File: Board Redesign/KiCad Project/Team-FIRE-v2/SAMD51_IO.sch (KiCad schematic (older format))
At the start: 20 parts, among them SW1 RESET, U5 SAMD51, U6 AT25DF041x-UxN-x, Y1 32.768kHz

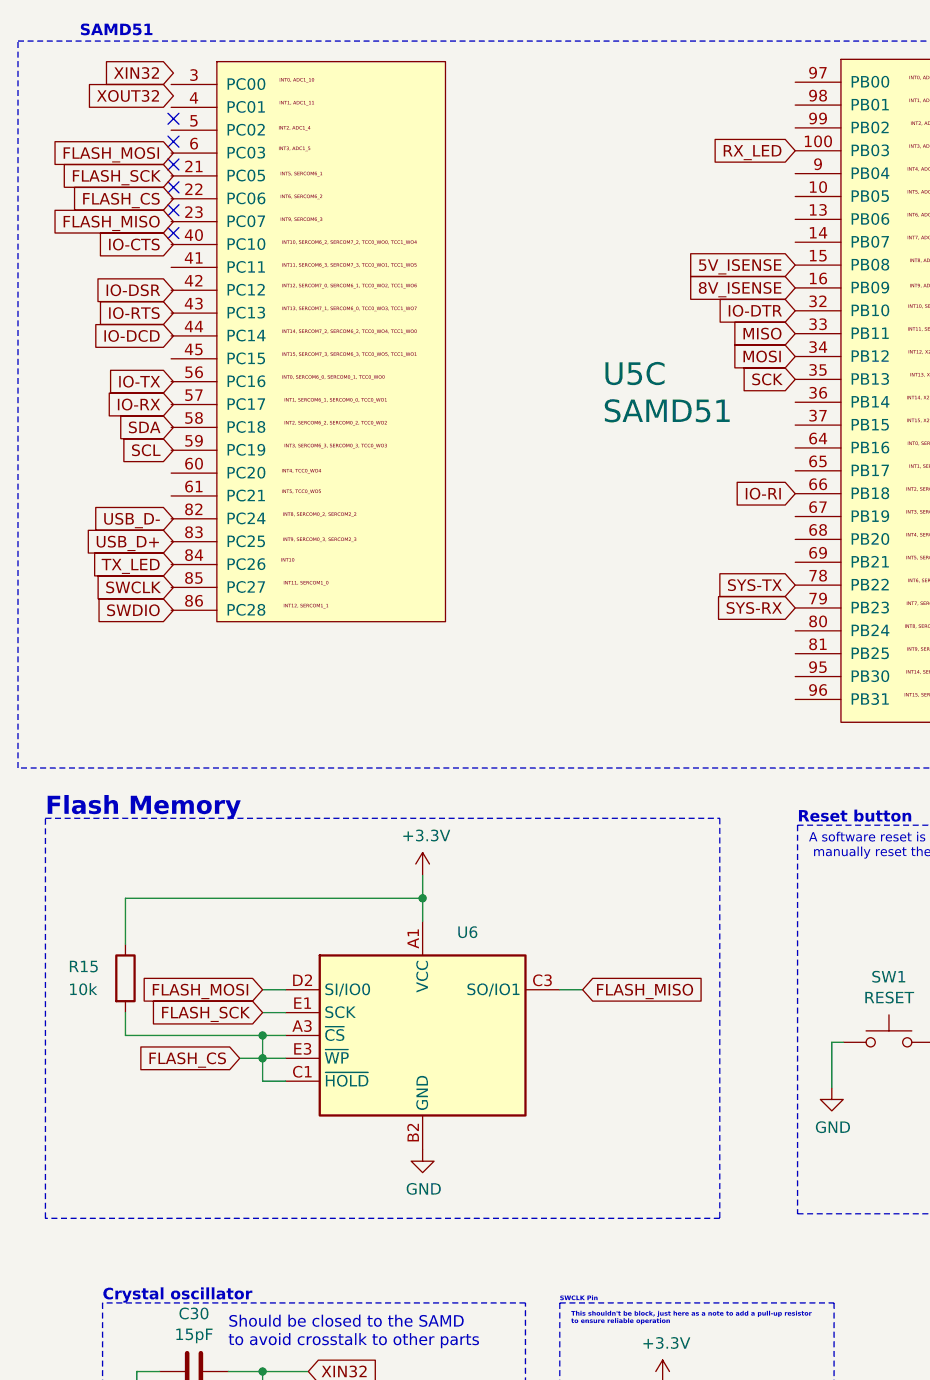
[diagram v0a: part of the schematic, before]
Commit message: Fixed some stuff (woops)
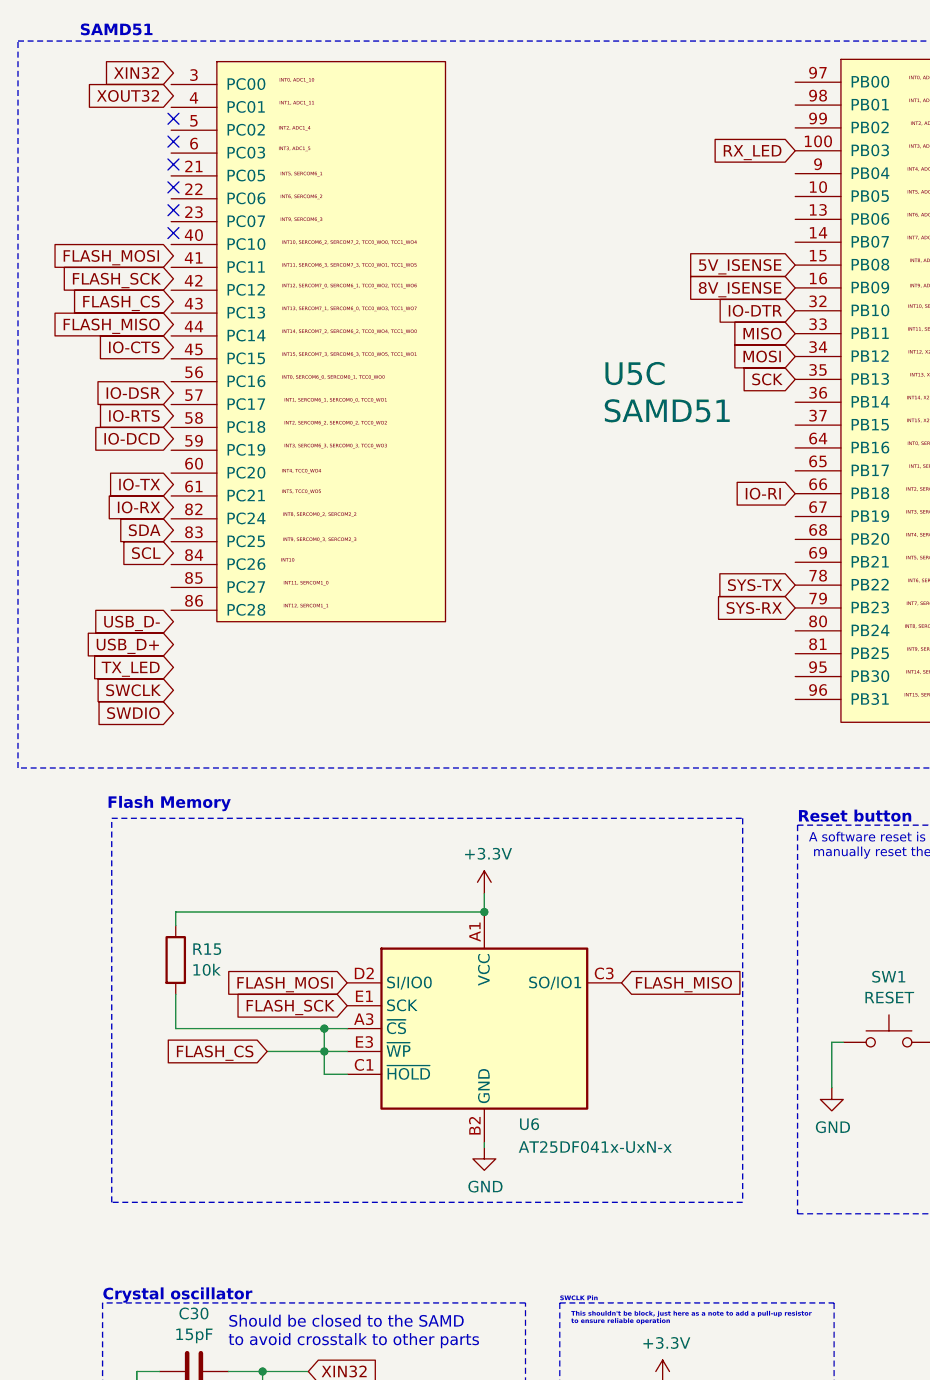
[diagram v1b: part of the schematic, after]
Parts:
- R15: footprint Resistor_SMD:R_0603_1608Metric -> (none); Link https://www.mouser.com/ProductDetail/Vishay-Beyschlag/MCT06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 -> (none); MPN MCT06030E1002BP100 -> (none); Manufacturer Vishay -> (none); Supplier Mouser -> (none); Supplier PN 594-MCT06030E1002BP1 -> (none); Tolerance 0.1% -> (none); Type Thin Film Resistor -> (none); Voltage Rating 75 V -> (none)
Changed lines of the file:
@@
 Comment4 ""
 $EndDescr
+Text GLabel 1260 3190 0    50   Input ~ 0
+USB_D-
+Text GLabel 1260 3290 0    50   Input ~ 0
+USB_D+
+Text GLabel 1260 2790 0    50   Input ~ 0
+SDA
+Text GLabel 1260 2890 0    50   Input ~ 0
+SCL
 $Comp
 L Team-FIRE:SAMD51 U?
@@
 	1    0    0    -1
 $EndComp
+Text GLabel 1260 3490 0    50   Input ~ 0
+SWCLK
+Text GLabel 1260 3590 0    50   Input ~ 0
+SWDIO
 Text GLabel 3980 1130 0    50   Input ~ 0
 RX_LED
+Text GLabel 1260 3390 0    50   Input ~ 0
+TX_LED
 Text GLabel 6740 3010 0    50   Input ~ 0
 SWO
@@
 Text Notes 6190 4060 0    50   ~ 10
 SAMD51 Power decoupling capacitors
-Text GLabel 3050 4800 2    50   Input ~ 0
+$Comp
+L Memory_Flash:AT25DF041x-UxN-x U?
+U 1 1 5F15C396
+P 2620 4970
+AR Path="/5E4F8378/5EA71818/5F15C396" Ref="U?"  Part="1"
+AR Path="/5E4F8378/5ED4DEFC/5ED7D75E/5F15C396" Ref="U?"  Part="1"
+AR Path="/5E4F8378/5ED4DEFC/5F15C396" Ref="U6"  Part="1"
+F 0 "U6" H 2770 4550 50  0000 L CNN
+F 1 "AT25DF041x-UxN-x" H 2770 4450 50  0000 L CNN
+F 2 "Package_CSP:WLCSP-8_1.58x1.63x0.35mm_Layout3x5_P0.35x0.4mm_Ball0.25mm_Pad0.25mm_NSMD" H 2420 4370 50  0001 C CNN
+F 3 "http://www.adestotech.com/wp-content/uploads/DS-AT25DF041B_040.pdf" H 2620 5670 50  0001 C CNN
+	1    2620 4970
+	1    0    0    -1
+$EndComp
+Text GLabel 3220 4770 2    50   Input ~ 0
 FLASH_MISO
+Text GLabel 2020 4870 0    50   Input ~ 0
+FLASH_SCK
+Text GLabel 2020 4770 0    50   Input ~ 0
+FLASH_MOSI
+Wire Wire Line
+	2620 5490 2620 5470
 $Comp
 L power:+3.3V #PWR?
 U 1 1 5F15C3A7
-P 2350 4300
+P 2620 4380
 AR Path="/5E4F8378/5EA71818/5F15C3A7" Ref="#PWR?"  Part="1"
 AR Path="/5E4F8378/5ED4DEFC/5ED7D75E/5F15C3A7" Ref="#PWR?"  Part="1"
 AR Path="/5E4F8378/5ED4DEFC/5F15C3A7" Ref="#PWR0138"  Part="1"
-F 0 "#PWR0138" H 2350 4150 50  0001 C CNN
-F 1 "+3.3V" H 2365 4473 50  0000 C CNN
-F 2 "" H 2350 4300 50  0001 C CNN
-F 3 "" H 2350 4300 50  0001 C CNN
-	1    2350 4300
-	1    0    0    -1
-$EndComp
+F 0 "#PWR0138" H 2620 4230 50  0001 C CNN
+F 1 "+3.3V" H 2635 4553 50  0000 C CNN
+F 2 "" H 2620 4380 50  0001 C CNN
+F 3 "" H 2620 4380 50  0001 C CNN
+	1    2620 4380
+	1    0    0    -1
+$EndComp
+Wire Wire Line
+	2620 4380 2620 4460
+Wire Wire Line
+	2020 4970 1920 4970
+Wire Wire Line
+	2020 5070 1920 5070
+Wire Wire Line
+	1920 5070 1920 4970
+Connection ~ 1920 4970
+Wire Wire Line
+	1920 5070 1670 5070
+Connection ~ 1920 5070
+Connection ~ 2620 4460
+Wire Wire Line
+	2620 4460 2620 4470
+Wire Wire Line
+	1270 4820 1270 4970
+Wire Wire Line
+	1270 4520 1270 4460
+Wire Wire Line
+	2020 5170 1920 5170
+Wire Wire Line
+	1920 5170 1920 5070
+Wire Wire Line
+	1270 4460 2620 4460
+Wire Wire Line
+	1270 4970 1920 4970
+Text Notes 970  4020 0    50   ~ 10
+Flash Memory
 $Comp
 L Device:Crystal Y?
@@
 Wire Notes Line
 	3990 4080 5940 4080
+Wire Notes Line
+	990  4050 3750 4050
+Wire Notes Line
+	3750 4050 3750 5730
+Wire Notes Line
+	3750 5730 990  5730
+Wire Notes Line
+	990  5730 990  4060
 Connection ~ 8620 4640
 Wire Wire Line
@@
 	8310 4510 8310 4640
 Connection ~ 8620 4510
+Text GLabel 1260 1590 0    50   Input ~ 0
+FLASH_MOSI
+Text GLabel 1260 1790 0    50   Input ~ 0
+FLASH_CS
+Text GLabel 1260 1890 0    50   Input ~ 0
+FLASH_MISO
+Text GLabel 1260 1690 0    50   Input ~ 0
+FLASH_SCK
+Text GLabel 1260 2290 0    50   Input ~ 0
+IO-RTS
+Text GLabel 1260 1990 0    50   Input ~ 0
+IO-CTS
+Text GLabel 1260 2190 0    50   Input ~ 0
+IO-DSR
+Text GLabel 1260 2390 0    50   Input ~ 0
+IO-DCD
 Text GLabel 3980 2630 0    50   Input ~ 0
 IO-RI
+Text GLabel 1260 2590 0    50   Input ~ 0
+IO-TX
+Text GLabel 1260 2690 0    50   Input ~ 0
+IO-RX
 Text GLabel 3980 1830 0    50   Input ~ 0
 IO-DTR
@@
 	1    0    0    -1
 $EndComp
+$Comp
+L Device:R R?
+U 1 1 5F15C3AE
+P 1270 4670
+AR Path="/5E4F8378/5EA71818/5F15C3AE" Ref="R?"  Part="1"
+AR Path="/5E4F8378/5ED4DEFC/5ED7D75E/5F15C3AE" Ref="R?"  Part="1"
+AR Path="/5E4F8378/5ED4DEFC/5F15C3AE" Ref="R15"  Part="1"
+F 0 "R15" H 1340 4716 50  0000 L CNN
+F 1 "10k" H 1340 4625 50  0000 L CNN
+F 2 "" V 1200 4670 50  0001 C CNN
+F 3 "~" H 1270 4670 50  0001 C CNN
+	1    1270 4670
+	1    0    0    -1
+$EndComp
 NoConn ~ 1260 990
 NoConn ~ 1260 1090
@@
 Text GLabel 1850 6470 2    50   Input ~ 0
 XIN32
-Wire Wire Line
-	1750 4800 1650 4800
-Text GLabel 1550 5100 0    50   Input ~ 0
+$Comp
+L power:GND #PWR?
+U 1 1 5F15C3A0
+P 2620 5490
+AR Path="/5E4F8378/5EA71818/5F15C3A0" Ref="#PWR?"  Part="1"
+AR Path="/5E4F8378/5ED4DEFC/5ED7D75E/5F15C3A0" Ref="#PWR?"  Part="1"
+AR Path="/5E4F8378/5ED4DEFC/5F15C3A0" Ref="#PWR0137"  Part="1"
+F 0 "#PWR0137" H 2620 5240 50  0001 C CNN
+F 1 "GND" H 2625 5317 50  0000 C CNN
+F 2 "" H 2620 5490 50  0001 C CNN
+F 3 "" H 2620 5490 50  0001 C CNN
+	1    2620 5490
+	1    0    0    -1
+$EndComp
+Text GLabel 1670 5070 0    50   Input ~ 0
 FLASH_CS
-Wire Wire Line
-	1750 5100 1650 5100
-Wire Wire Line
-	1750 5200 1650 5200
-Wire Wire Line
-	1650 5000 1750 5000
-Wire Wire Line
-	1650 5000 1650 5100
-Connection ~ 1650 5100
-Wire Wire Line
-	1650 5100 1550 5100
-Wire Wire Line
-	1650 5100 1650 5200
-Wire Wire Line
-	2350 4300 2350 4400
-Wire Wire Line
-	2950 4800 3050 4800
-$Comp
-L power:GND #PWR?
-U 1 1 5EBDC8BA
-P 2350 5500
-AR Path="/5E4F8378/5EA71818/5EBDC8BA" Ref="#PWR?"  Part="1"
-AR Path="/5E4F8378/5ED4DEFC/5ED7D75E/5EBDC8BA" Ref="#PWR?"  Part="1"
-AR Path="/5E4F8378/5ED4DEFC/5EBDC8BA" Ref="#PWR013"  Part="1"
-F 0 "#PWR013" H 2350 5250 50  0001 C CNN
-F 1 "GND" H 2355 5327 50  0000 C CNN
-F 2 "" H 2350 5500 50  0001 C CNN
-F 3 "" H 2350 5500 50  0001 C CNN
-	1    2350 5500
-	1    0    0    -1
-$EndComp
-Wire Wire Line
-	1650 4900 1750 4900
-Text GLabel 1650 4900 0    50   Input ~ 0
-FLASH_SCK
-Text GLabel 1650 4800 0    50   Input ~ 0
-FLASH_MOSI
-$Comp
-L Device:R R?
-U 1 1 5EBDEFB3
-P 1050 4750
-AR Path="/5E4F8378/5EBDEFB3" Ref="R?"  Part="1"
-AR Path="/5E4F8378/5ED4DEFC/5EBDEFB3" Ref="R15"  Part="1"
-F 0 "R15" H 800 4800 50  0000 L CNN
-F 1 "10k" H 800 4700 50  0000 L CNN
-F 2 "Resistor_SMD:R_0603_1608Metric" V 980 4750 50  0001 C CNN
-F 3 "https://www.mouser.com/datasheet/2/427/mcx0x0xpre-1762843.pdf" H 1050 4750 50  0001 C CNN
-F 4 "MCT06030E1002BP100" H 1050 4750 50  0001 C CNN "MPN"
-F 5 "Vishay" H 1050 4750 50  0001 C CNN "Manufacturer"
-F 6 "Mouser" H 1050 4750 50  0001 C CNN "Supplier"
-F 7 "594-MCT06030E1002BP1" H 1050 4750 50  0001 C CNN "Supplier PN"
-F 8 "https://www.mouser.com/ProductDetail/Vishay-Beyschlag/MCT06030E1002BP100?qs=sGAEpiMZZMtlubZbdhIBIHIEm3drdiPa32EPxwxqfD0%3D" H 1050 4750 50  0001 C CNN "Link"
-F 9 "Thin Film Resistor" H 1050 4750 50  0001 C CNN "Type"
-F 10 "0.1%" H 1050 4750 50  0001 C CNN "Tolerance"
-F 11 "75 V" H 1050 4750 50  0001 C CNN "Voltage Rating"
-	1    1050 4750
-	1    0    0    -1
-$EndComp
-Wire Wire Line
-	1650 5000 1050 5000
-Wire Wire Line
-	1050 5000 1050 4900
-Connection ~ 1650 5000
-Wire Wire Line
-	1050 4600 1050 4400
-Wire Wire Line
-	1050 4400 2350 4400
-Connection ~ 2350 4400
-Wire Wire Line
-	2350 4400 2350 4500
-Wire Notes Line
-	700  4050 3650 4050
-Wire Notes Line
-	3650 4050 3650 5800
-Wire Notes Line
-	3650 5800 700  5800
-Wire Notes Line
-	700  5800 700  4050
-Text Notes 700  4050 0    79   ~ 16
-Flash Memory
-$Comp
-L Memory_Flash:AT25DF041x-UxN-x U6
-U 1 1 5EBC3761
-P 2350 5000
-F 0 "U6" H 2500 5450 50  0000 L CNN
-F 1 "AT25DF041x-UxN-x" H 2994 4955 50  0001 L CNN
-F 2 "Package_CSP:WLCSP-8_1.58x1.63x0.35mm_Layout3x5_P0.35x0.4mm_Ball0.25mm_Pad0.25mm_NSMD" H 2150 4400 50  0001 C CNN
-F 3 "http://www.adestotech.com/wp-content/uploads/DS-AT25DF041B_040.pdf" H 2350 5700 50  0001 C CNN
-	1    2350 5000
-	1    0    0    -1
-$EndComp
-Text GLabel 1260 2740 0    50   Input ~ 0
-USB_D-
-Text GLabel 1260 2840 0    50   Input ~ 0
-USB_D+
-Text GLabel 1260 2340 0    50   Input ~ 0
-SDA
-Text GLabel 1260 2440 0    50   Input ~ 0
-SCL
-Text GLabel 1260 3040 0    50   Input ~ 0
-SWCLK
-Text GLabel 1260 3140 0    50   Input ~ 0
-SWDIO
-Text GLabel 1260 2940 0    50   Input ~ 0
-TX_LED
-Text GLabel 1260 1140 0    50   Input ~ 0
-FLASH_MOSI
-Text GLabel 1260 1340 0    50   Input ~ 0
-FLASH_CS
-Text GLabel 1260 1440 0    50   Input ~ 0
-FLASH_MISO
-Text GLabel 1260 1240 0    50   Input ~ 0
-FLASH_SCK
-Text GLabel 1260 1840 0    50   Input ~ 0
-IO-RTS
-Text GLabel 1260 1540 0    50   Input ~ 0
-IO-CTS
-Text GLabel 1260 1740 0    50   Input ~ 0
-IO-DSR
-Text GLabel 1260 1940 0    50   Input ~ 0
-IO-DCD
-Text GLabel 1260 2140 0    50   Input ~ 0
-IO-TX
-Text GLabel 1260 2240 0    50   Input ~ 0
-IO-RX
 $EndSCHEMATC
